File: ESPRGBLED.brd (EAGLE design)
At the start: 22.5 x 22.9 mm, 24 parts

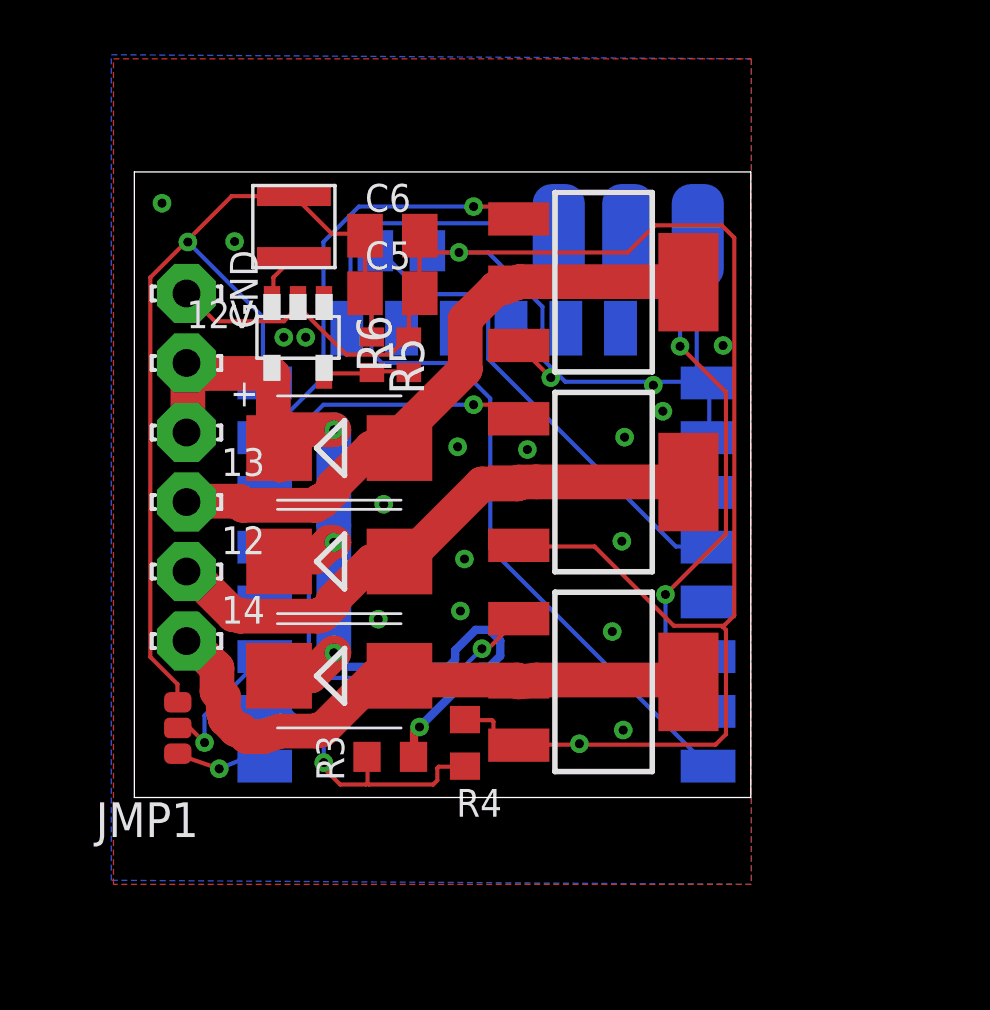
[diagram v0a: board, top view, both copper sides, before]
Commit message: layout stuff
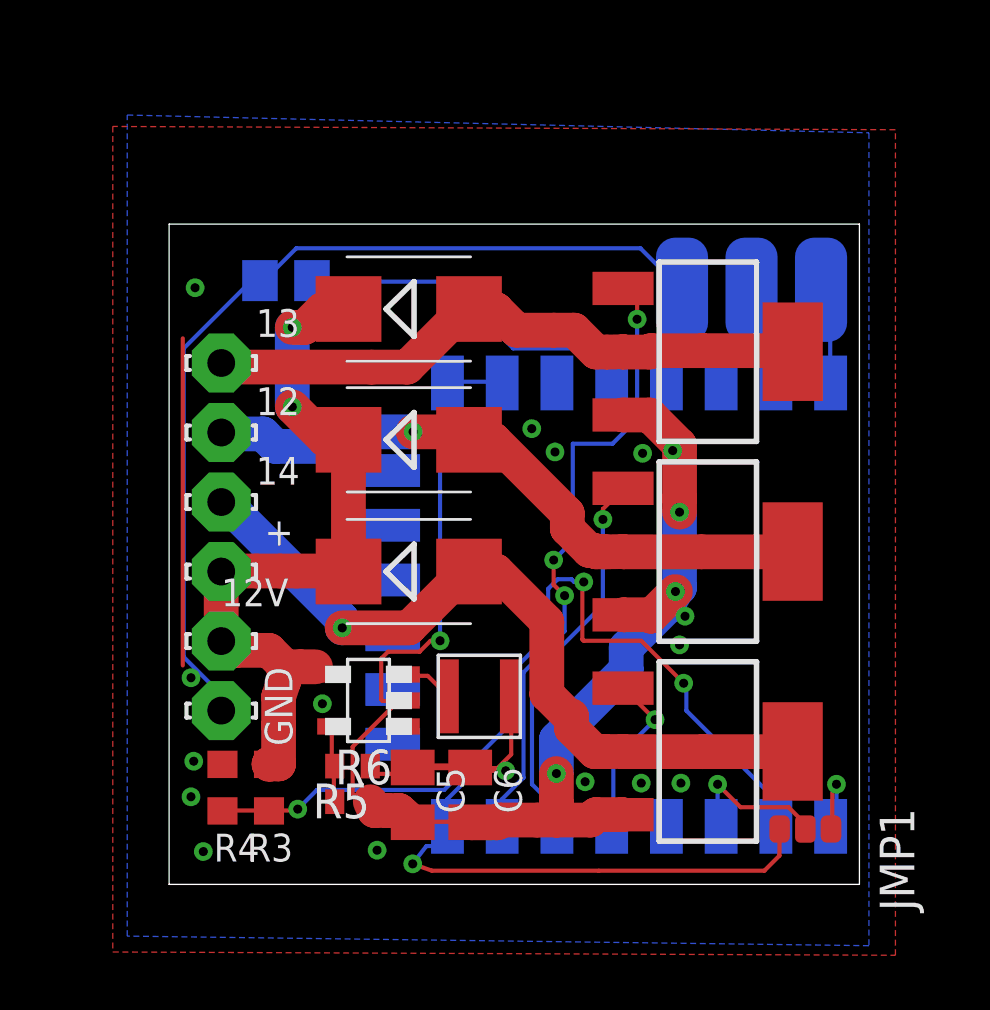
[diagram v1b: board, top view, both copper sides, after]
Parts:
- moved JMP1 23.2 mm to (23.2, 2.02), turned to 270 degrees
- moved C6 20.6 mm to (11.0, 3.27), turned to 270 degrees
- moved MDL1 18.8 mm to (8.17, 2.12), turned to 90 degrees
- moved L1 18.5 mm to (11.3, 6.87), turned to 0 degrees
- moved C5 18.3 mm to (8.90, 3.27), turned to 270 degrees
- moved R6 16.5 mm to (6.70, 3.02), turned to 0 degrees
- moved GND 15.3 mm to (1.91, 6.35)
- moved R5 15.0 mm to (6.70, 4.32), turned to 180 degrees
- moved U$2 13.5 mm to (7.29, 6.72), turned to 90 degrees
- moved 12V 10.2 mm to (1.91, 8.89)
- moved R4 9.01 mm to (1.95, 3.54)
- moved PWR1:D1 5.68 mm to (8.76, 21.0)
- moved + 5.24 mm to (1.91, 11.4)
- moved 12 5.24 mm to (1.91, 16.5)
- moved 13 5.24 mm to (1.91, 19.1)
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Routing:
- net N$7: track 34.5 -> 3.56 mm
- net N$10: track 10.5 -> 32.0 mm, vias 1 -> 3
- net N$8: track 20.4 -> 3.81 mm, vias 2 -> 0
- net GND: track 87.7 -> 99.1 mm
- net +12V: track 37.5 -> 27.6 mm, vias 4 -> 2
- net N$6: track 15.9 -> 23.4 mm, vias 1 -> 3
- net N$2: track 13.7 -> 6.22 mm
- net N$5: track 21.8 -> 28.3 mm, vias 0 -> 1
- net N$9: track 17.8 -> 12.5 mm
- net VCC: track 35.8 -> 32.0 mm, vias 1 -> 2
- net N$3: track 11.5 -> 14.1 mm
- net N$4: track 21.1 -> 23.4 mm, vias 0 -> 1
- net N$15: track 3.16 -> 3.89 mm
- net N$1: track 23.2 -> 22.5 mm
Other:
- board size 22.5 x 22.9 mm -> 25.2 x 24.1 mm

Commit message: superminiaturized
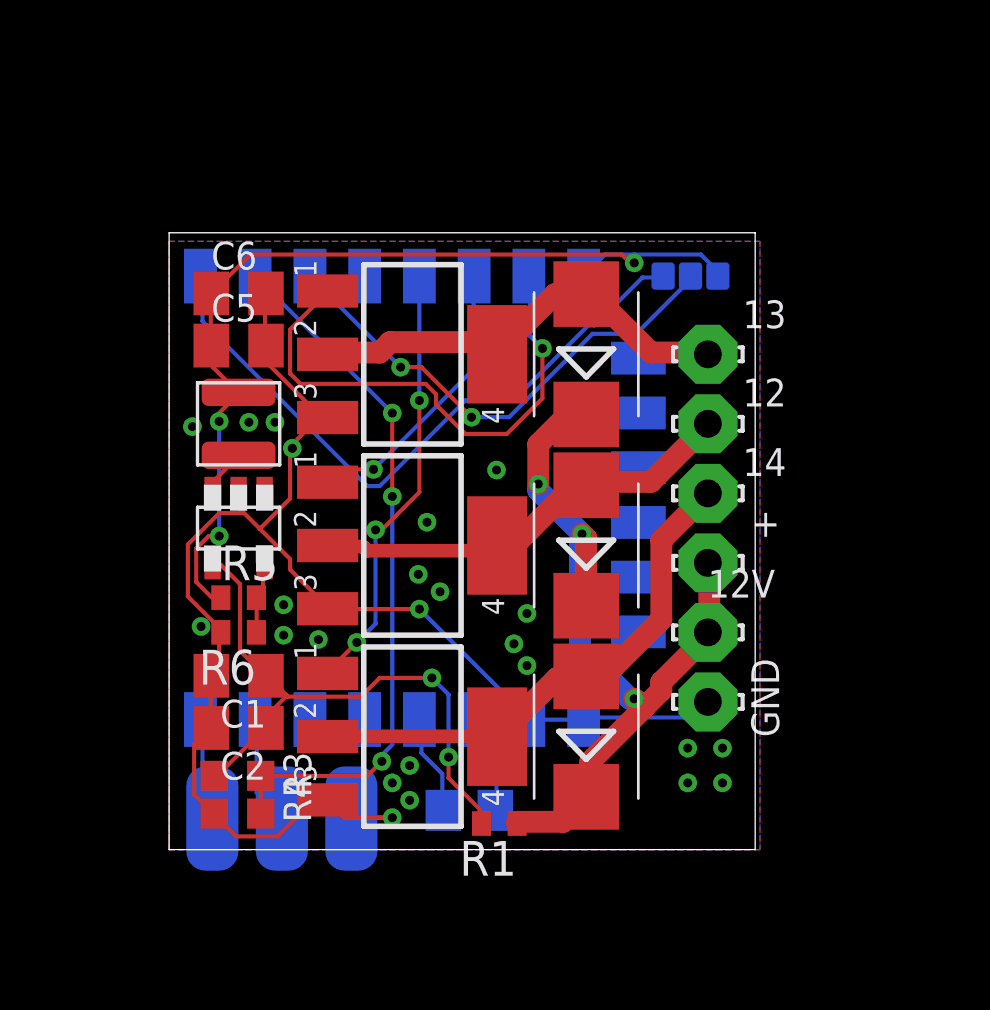
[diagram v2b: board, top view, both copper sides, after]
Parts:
- added C1, C2: 10uF, rcl:C0805K
- added R1: 0R, rcl:R0402
- R5: value (none) -> 61k9
- R6: value (none) -> 20k
- moved U$3 25.8 mm to (4.12, 2.40), turned to 0 degrees
- moved MDL1 22.0 mm to (17.1, 22.2), turned to 270 degrees
- moved JMP1 20.6 mm to (19.1, 22.2), flipped to the bottom
- moved R2 20.5 mm to (11.0, 2.71), turned to 180 degrees
- moved C6 20.2 mm to (2.54, 21.6), turned to 0 degrees
- moved + 17.8 mm to (19.7, 11.7)
- moved 12 17.8 mm to (19.7, 16.8)
- moved 12V 17.8 mm to (19.7, 9.21)
- moved 13 17.8 mm to (19.7, 19.4)
- moved 14 17.8 mm to (19.7, 14.3)
- moved GND 17.8 mm to (19.7, 6.67)
- moved C5 17.6 mm to (2.54, 19.7), turned to 0 degrees
- moved L1 13.3 mm to (2.54, 16.8), turned to 90 degrees
- moved PWR3:T1 10.8 mm to (8.89, 5.40)
- moved PWR2:T1 10.8 mm to (8.89, 12.4)
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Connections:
- net N$10 renamed ADC
- net N$11 renamed REST
- net N$12 renamed CH_PD
- net N$2 renamed GPIO14
- net N$3 renamed GPIO12
- net N$6 renamed GPIO13
- net N$9 renamed GPIO0
- new net VIN: C1.1, C2.1, R1.2, R3.2, U$2.4
- net +12V: now also R1.1; no longer R3.2, U$2.4
- net GND: now also C1.2, C2.2
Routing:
- net GND: track 99.1 -> 59.2 mm, vias 20 -> 24
- net VIN: track 0.00 -> 21.9 mm, vias 0 -> 2
- net REST: track 3.37 -> 24.2 mm, vias 1 -> 0
- net CH_PD: track 5.60 -> 18.3 mm, vias 1 -> 2
- net GPIO14: track 6.22 -> 16.0 mm, vias 1 -> 3
- net N$5: track 28.3 -> 19.3 mm, vias 1 -> 0
- net GPIO0: track 12.5 -> 3.72 mm
- net N$4: track 23.4 -> 15.9 mm, vias 1 -> 0
- net N$1: track 22.5 -> 16.2 mm
- net ADC: track 32.0 -> 26.0 mm
- net GPIO13: track 23.4 -> 19.1 mm, vias 3 -> 1
- net GPIO12: track 14.1 -> 10.5 mm
- net VCC: track 32.0 -> 35.1 mm, vias 2 -> 3
- net +12V: track 27.6 -> 29.9 mm, vias 2 -> 3
- net N$15: track 3.89 -> 2.61 mm
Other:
- board size 25.2 x 24.1 mm -> 21.4 x 22.5 mm
